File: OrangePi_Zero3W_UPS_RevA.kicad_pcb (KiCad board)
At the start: 4 copper layers, 65 x 32 mm, 9 parts, among them J1 ORANGE_PI_ZERO_3W_HEADER, U1 MAX17048G_T10

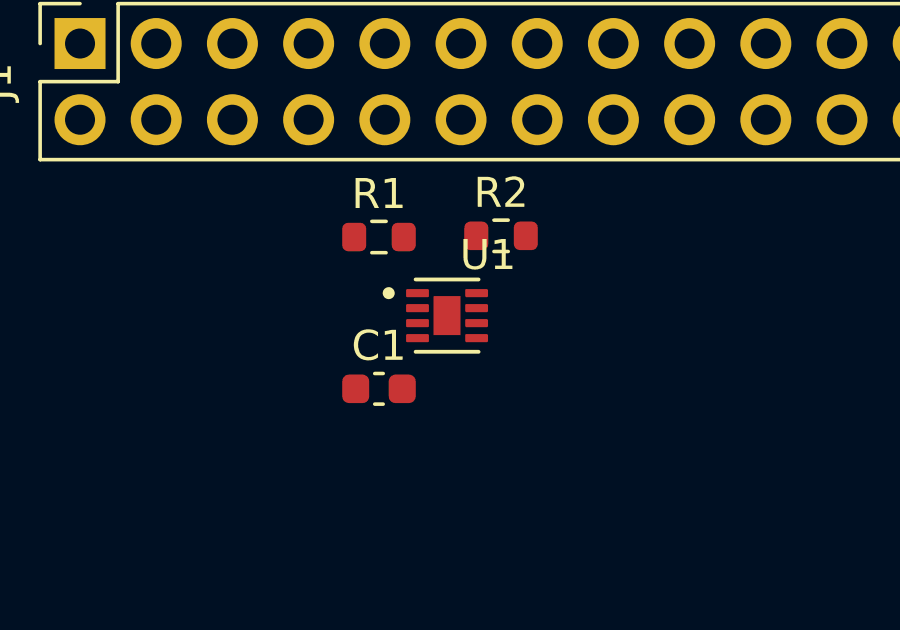
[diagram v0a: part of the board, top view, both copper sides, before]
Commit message: phase 5B.1B
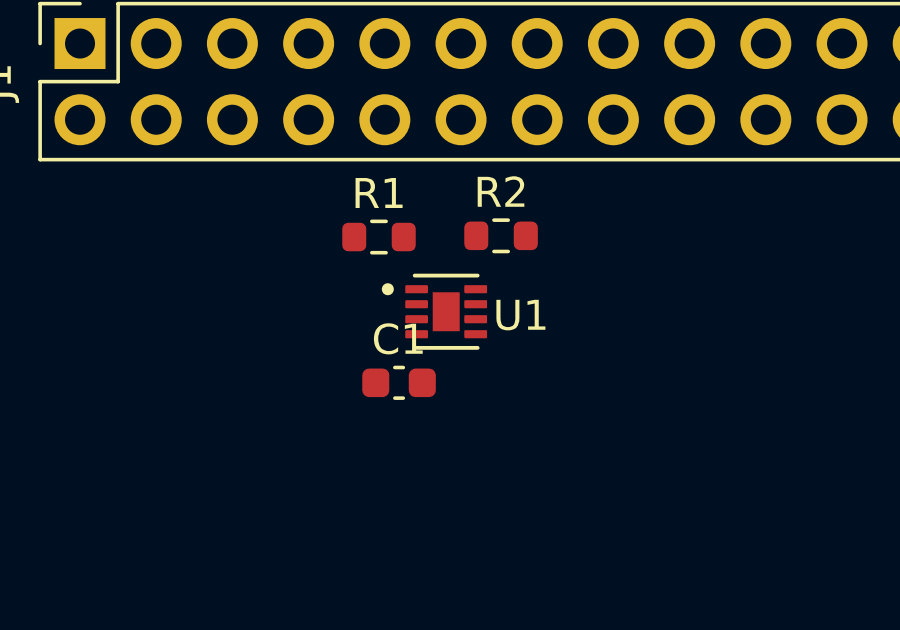
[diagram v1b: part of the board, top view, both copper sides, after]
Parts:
- moved C1 0.70 mm to (74.6, 86.2)
- moved U1 0.13 mm to (76.2, 83.8)
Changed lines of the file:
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@@
 	(footprint "Capacitor_SMD:C_0603_1608Metric"
 		(layer "F.Cu")
-		(at 73.975 86.38)
+		(at 74.645 86.18)
 		(descr "Capacitor SMD 0603 (1608 Metric), square (rectangular) end terminal, IPC-7351 nominal, (Body size source: IPC-SM-782 page 76, https://www.pcb-3d.com/wordpress/wp-content/uploads/ipc-sm-782a_amendment_1_and_2.pdf), generated with kicad-footprint-generator")
 		(tags "capacitor")
@@
 	(footprint "MAX17048G_T10:SON50P200X200X80-9N"
 		(layer "F.Cu")
-		(at 76.245 83.94)
+		(at 76.215 83.81)
 		(property "Reference" "U1"
-			(at 1.365 -2.017 0)
-			(layer "F.SilkS")
-			(effects
+			(at 2.495 0.14 0)
+			(layer "F.SilkS")
+			(effects
